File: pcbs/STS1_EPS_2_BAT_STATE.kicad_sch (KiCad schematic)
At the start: 5 parts, among them U3 MIC841

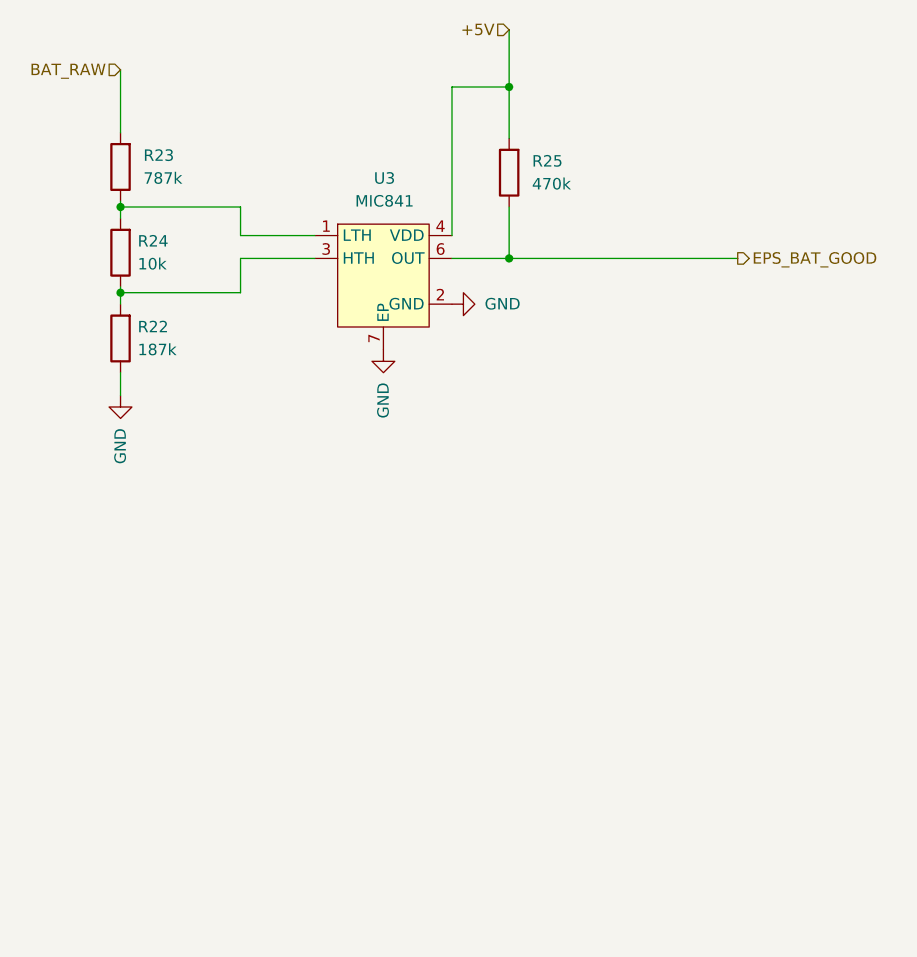
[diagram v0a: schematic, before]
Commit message: worked on sts1_eps_1
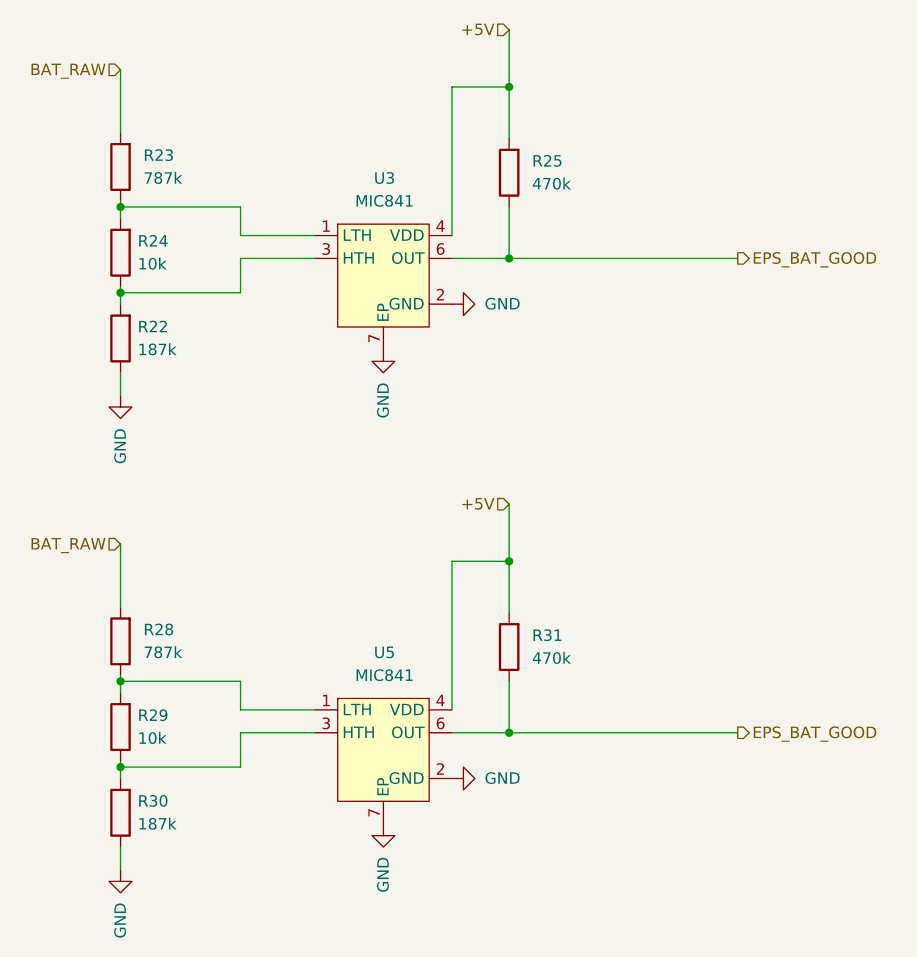
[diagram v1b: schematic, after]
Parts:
- added R28: 787k, Resistor_SMD:R_0805_2012Metric, symbol Device:R
- added R29: 10k, Resistor_SMD:R_0805_2012Metric, symbol Device:R
- added R30: 187k, Resistor_SMD:R_0805_2012Metric, symbol Device:R
- added R31: 470k, Resistor_SMD:R_0805_2012Metric, symbol Device:R
- added U5: MIC841, Package_DFN_QFN:TDFN-6-1EP_2.5x2.5mm_P0.65mm_EP1.3x2mm, symbol STS_Analog:MIC841
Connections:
- net +5V: now also R31.2, U5.4 (VDD)
- net BAT_RAW: now also R28.2
- net EPS_BAT_GOOD: now also R31.1, U5.6 (OUT)
- net GND: now also R30.1, U5.2 (GND), U5.7 (EP)
- new net: R28.1, R29.2, U5.1 (LTH)
- new net: R29.1, R30.2, U5.3 (HTH)
